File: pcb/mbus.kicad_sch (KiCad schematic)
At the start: 25 parts, among them Q3 BSS84, Q5 Q_NPN_BEC_BRT, U3 MC33072, U4 LM4040DBZ-5

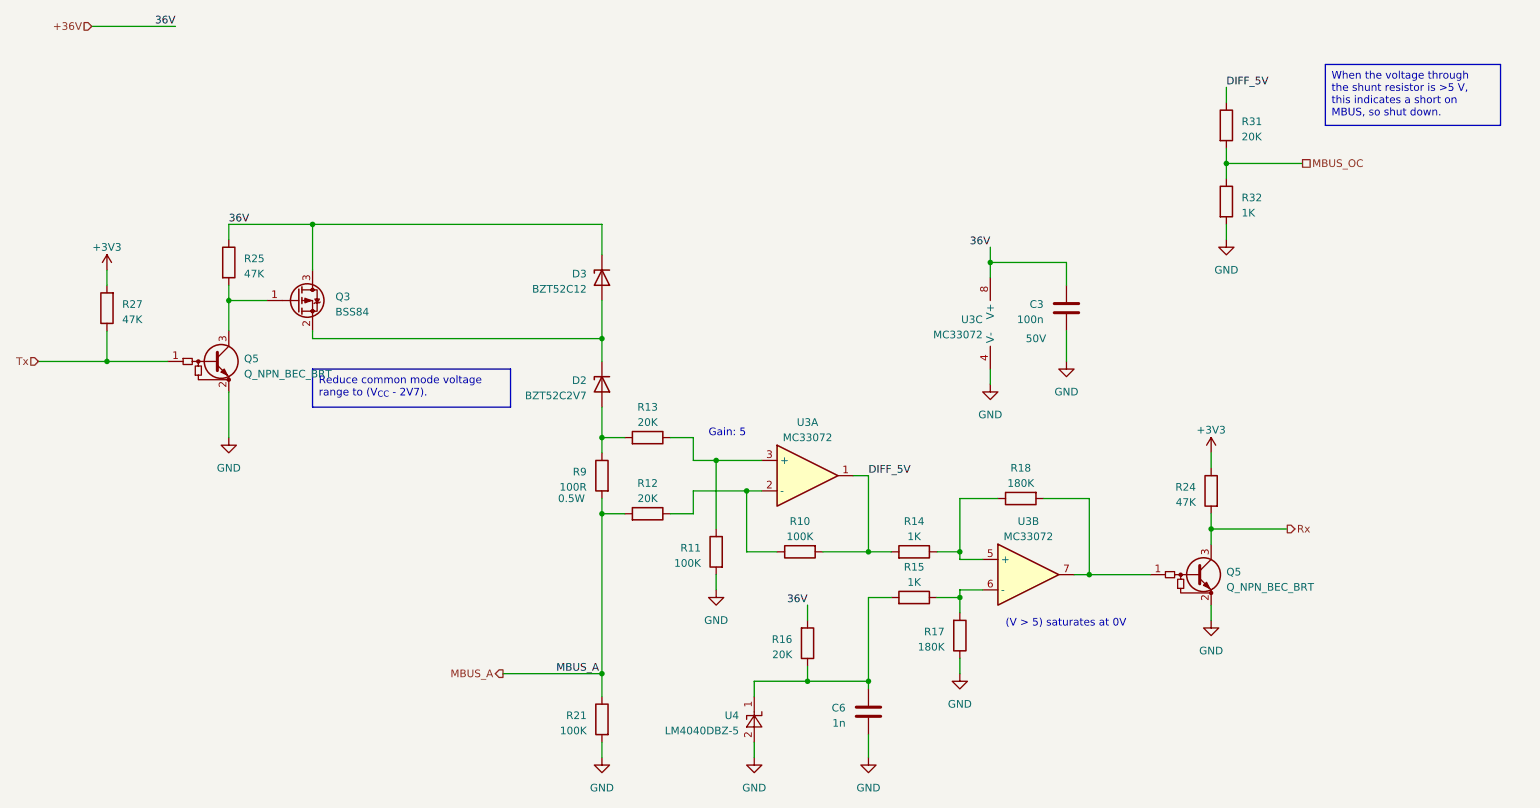
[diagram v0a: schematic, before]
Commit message: [v0.1-dev] First pass on emonPi format
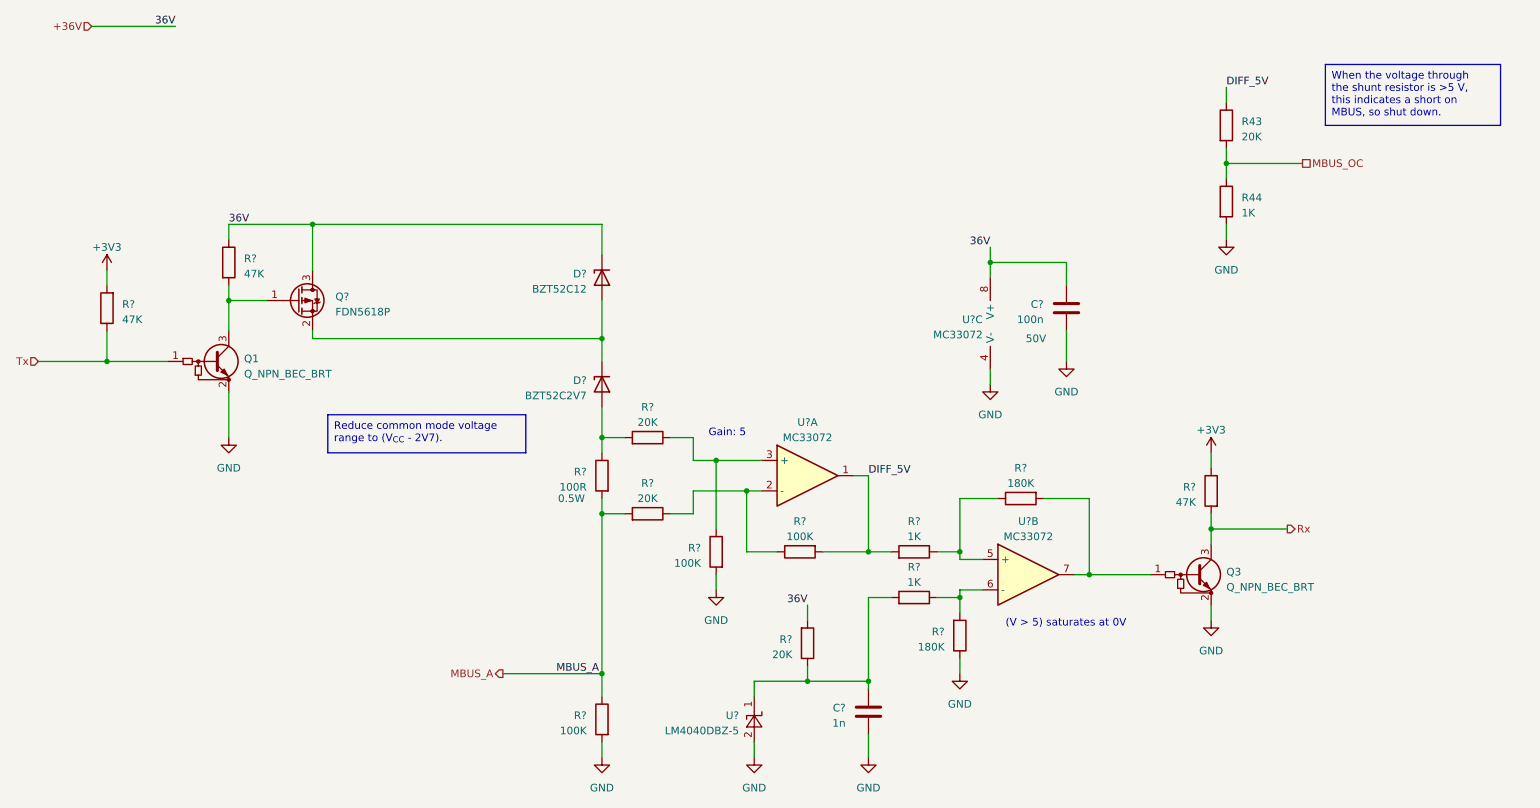
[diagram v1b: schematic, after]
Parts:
- Q?: renamed from Q3; value BSS84 -> FDN5618P
- U? (x3): renamed from U3; MPN (none) -> MC33072DR2G; Mouser (none) -> 863-MC33072DR2G
- U?: renamed from U4; MPN (none) -> LM4040DYM3-5.0-TR; Mouser (none) -> 998-LM4040DYM3-5.0TR
- renumbered C6 to C?, C3 to C?, D3 to D?, D2 to D?, Q5 to Q1, Q5 to Q3, R31 to R43, R32 to R44, R25 to R?, R24 to R?, R14 to R?, R21 to R?, R13 to R?, R18 to R?, R16 to R?, R17 to R?, R27 to R?, R12 to R?, R11 to R?, R9 to R?, R10 to R?, R15 to R?
